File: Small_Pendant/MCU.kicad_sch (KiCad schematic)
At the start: 17 parts, among them U2 SN74LVC1T45DCK

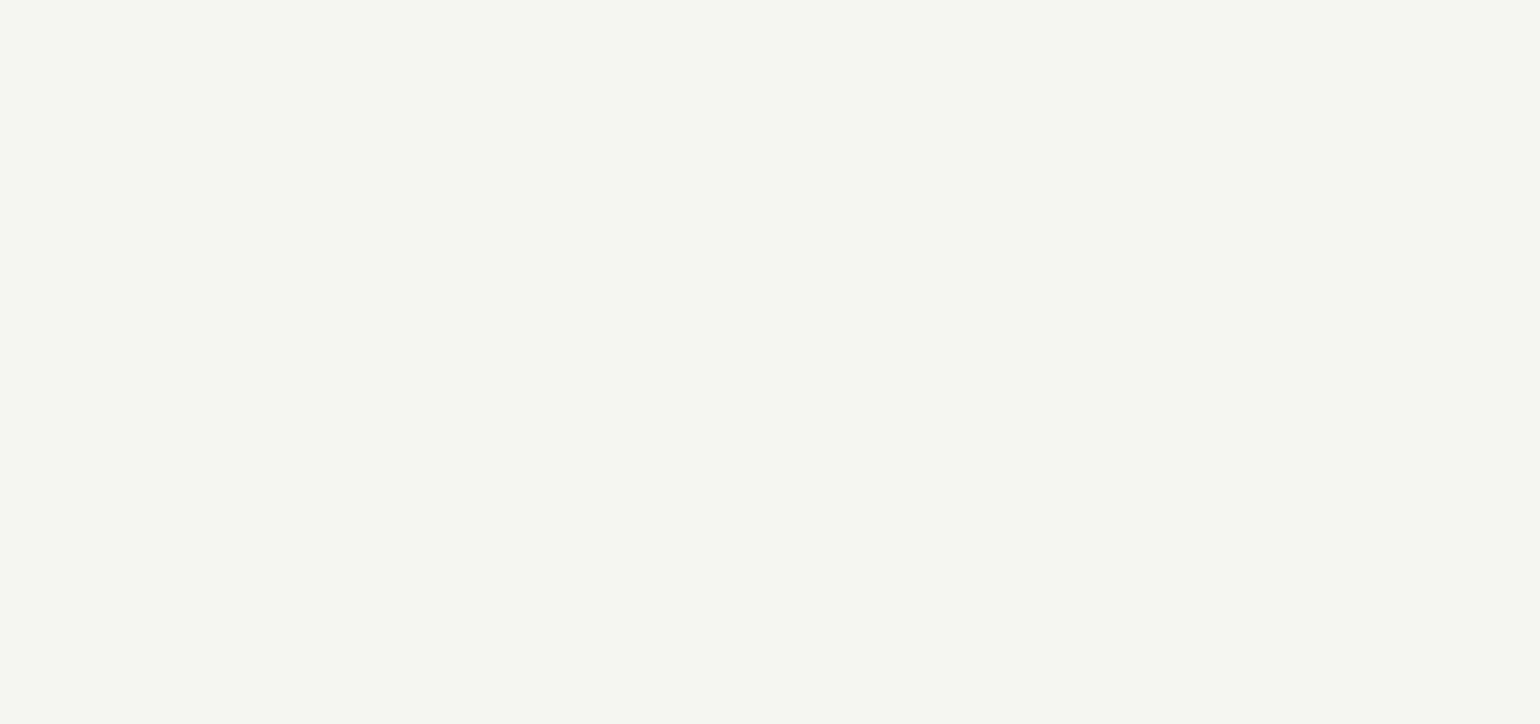
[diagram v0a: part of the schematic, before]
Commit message: [HW] Update TODOs and combine USB Power Rails
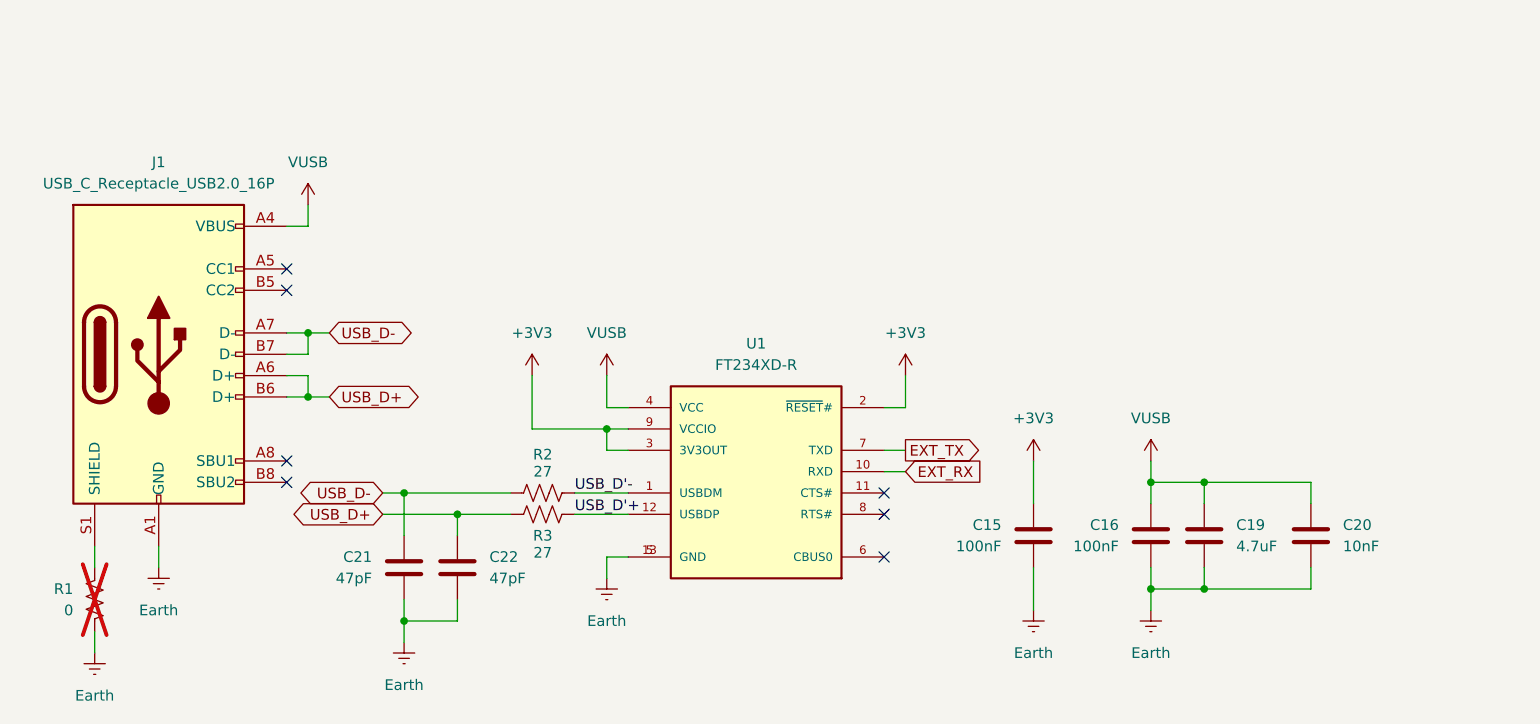
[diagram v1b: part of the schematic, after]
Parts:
- added C15, C16: 100nF, Capacitor_SMD:C_0402_1005Metric, symbol Device:C
- added C19: 4.7uF, Capacitor_SMD:C_0402_1005Metric, symbol Device:C
- added C20: 10nF, Capacitor_SMD:C_0402_1005Metric, symbol Device:C
- added C21, C22: 47pF, Capacitor_SMD:C_0402_1005Metric, symbol Device:C
- added J1: USB_C_Receptacle_USB2.0_16P, Connector_USB:USB_C_Receptacle_GCT_USB4105-xx-A_16P_TopMnt_Horizontal, symbol Connector:USB_C_Receptacle_USB2.0_16P
- added R1: 0, Resistor_SMD:R_0402_1005Metric, symbol Device:R_US
- added R2, R3: 27, Resistor_SMD:R_0402_1005Metric, symbol Device:R_US
- added U1: FT234XD-R, Package_DFN_QFN:DFN-12-1EP_3x3mm_P0.45mm_EP1.65x2.38mm, symbol Interface_USB:FT234XD-R
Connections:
- net +3V3: now also C15.1, U1.2 (~{RESET}#), U1.3 (3V3OUT), U1.9 (VCCIO)
- net Earth: now also C15.2, C16.2, C19.2, C20.2, C21.2, C22.2, J1.A1 (GND), J1.A12 (GND), J1.B1 (GND), J1.B12 (GND), R1.1, U1.13 (GND), U1.5 (GND)
- new net: J1.S1 (SHIELD), R1.2
- new net EXT_RX: U1.10 (RXD)
- new net EXT_TX: U1.7 (TXD)
- new net USB_D'+: R3.2, U1.12 (USBDP)
- new net USB_D'-: R2.2, U1.1 (USBDM)
- new net USB_D+: C22.1, J1.A6 (D+), J1.B6 (D+), R3.1
- new net USB_D-: C21.1, J1.A7 (D-), J1.B7 (D-), R2.1
- new net VUSB: C16.1, C19.1, C20.1, J1.A4 (VBUS), J1.A9 (VBUS), J1.B4 (VBUS), J1.B9 (VBUS), U1.4 (VCC)
- no-connect marks 0 -> 7

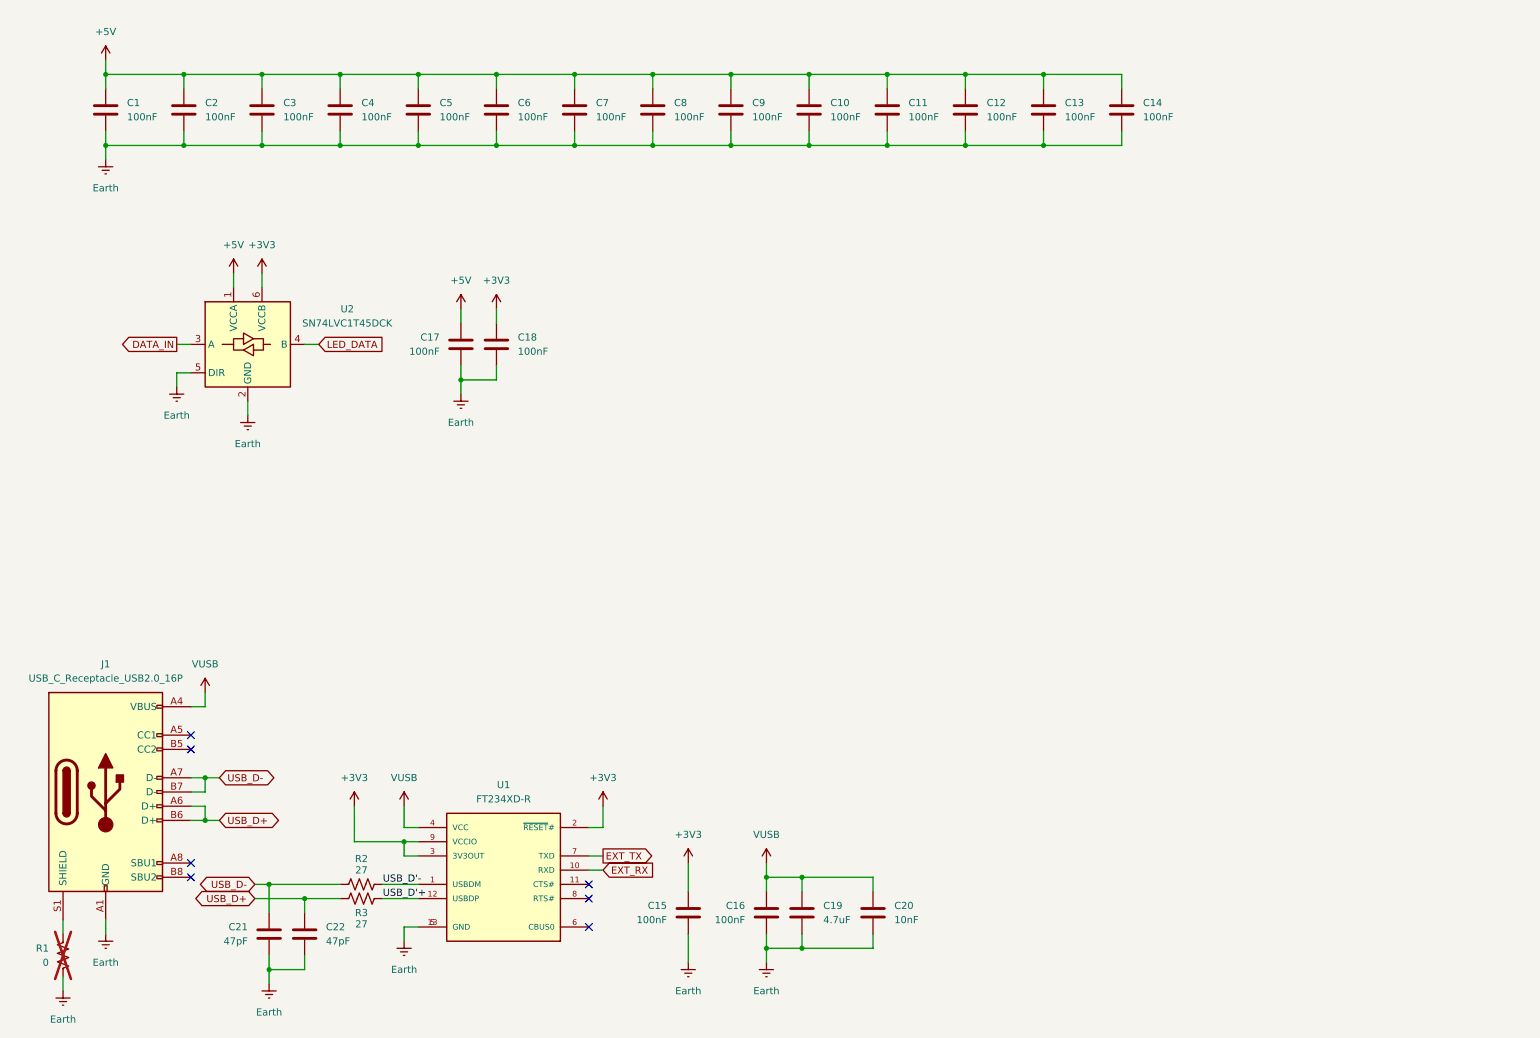
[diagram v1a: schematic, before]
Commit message: [HW] Remove Blind Vias, add 5k1 CC resistors for 5V3A USB-C TODO: 3V3 Regulator (May switch FTDI to that) TODO: MCU (OSC?)
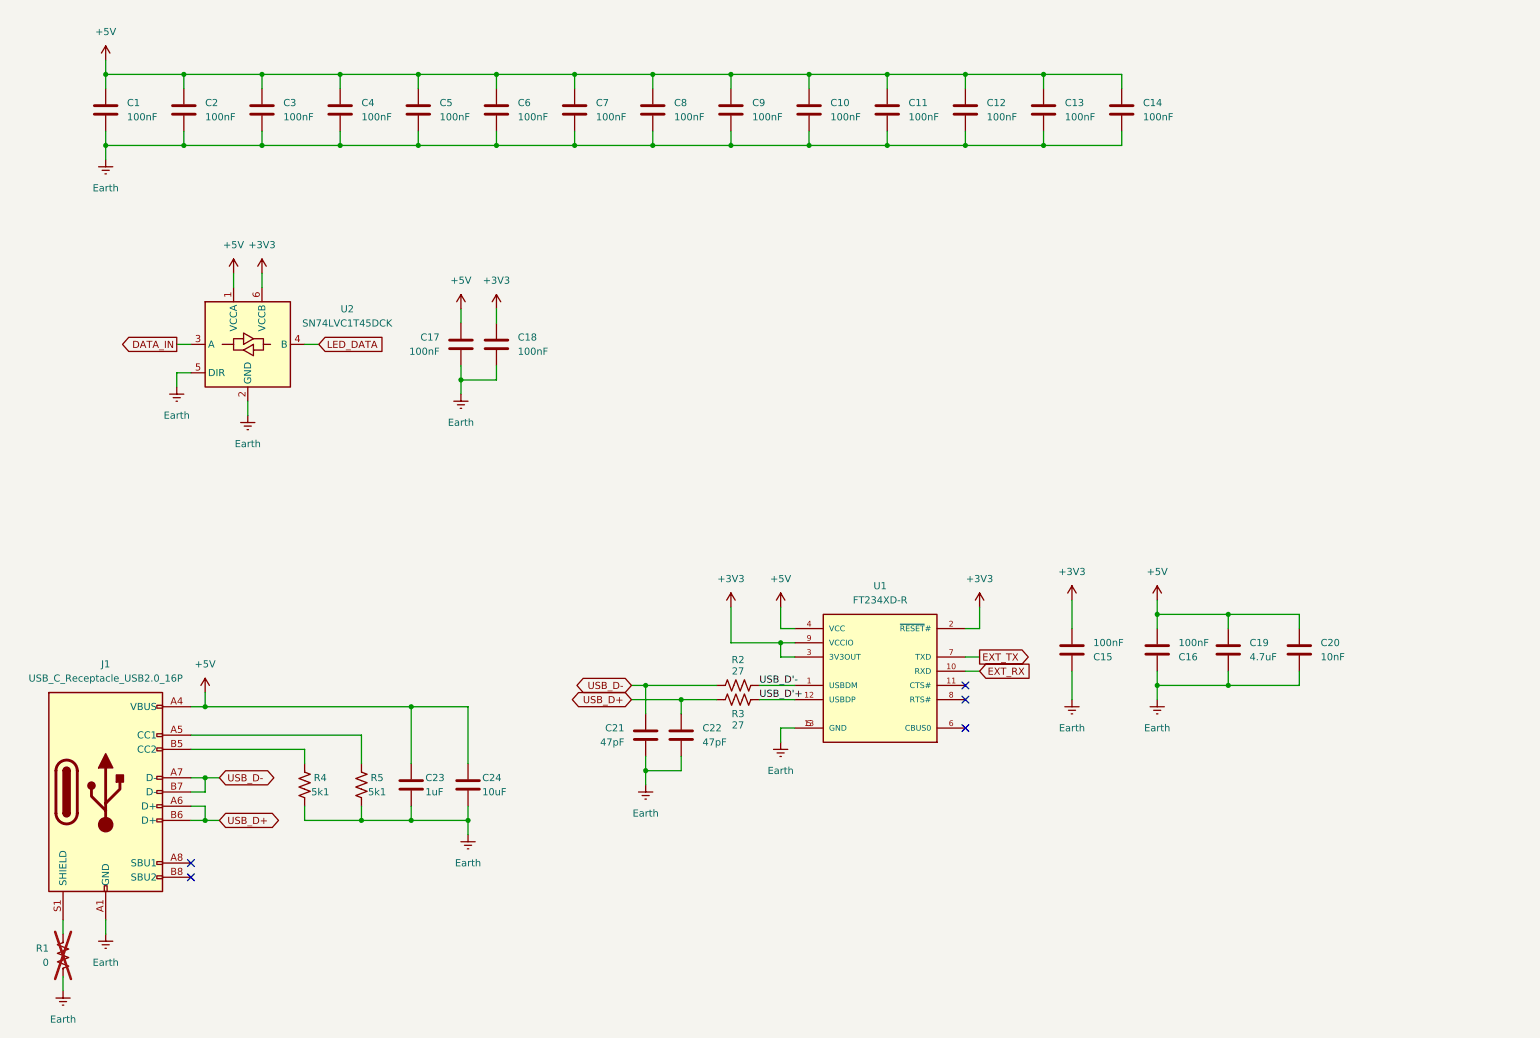
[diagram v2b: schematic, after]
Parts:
- added C23: 1uF, Capacitor_SMD:C_0402_1005Metric, symbol Device:C
- added C24: 10uF, Capacitor_SMD:C_0402_1005Metric, symbol Device:C
- added R4, R5: 5k1, Resistor_SMD:R_0402_1005Metric, symbol Device:R_US
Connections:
- net +3V3: now also C15.2; no longer C15.1
- net +5V: now also C16.2, C19.1, C20.1, J1.A4 (VBUS), J1.A9 (VBUS), J1.B4 (VBUS), J1.B9 (VBUS), U1.4 (VCC), C23.1, C24.1
- net Earth: now also C15.1, C16.1, C23.2, C24.2, R4.2, R5.2; no longer C15.2, C16.2
- net at J1.A5 (CC1): now also R5.1
- net at J1.B5 (CC2): now also R4.1
- removed net VUSB: C16.1, C19.1, C20.1, J1.A4 (VBUS), J1.A9 (VBUS), J1.B4 (VBUS), J1.B9 (VBUS), U1.4 (VCC)
- no-connect marks 7 -> 5
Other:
- moved on the sheet: C15, C16, C19, C20, C21, C22, R2, R3, U1

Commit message: [HW] Split Boards, need to move Caps for LEDs and add all the assorcted stuff for the ESP32
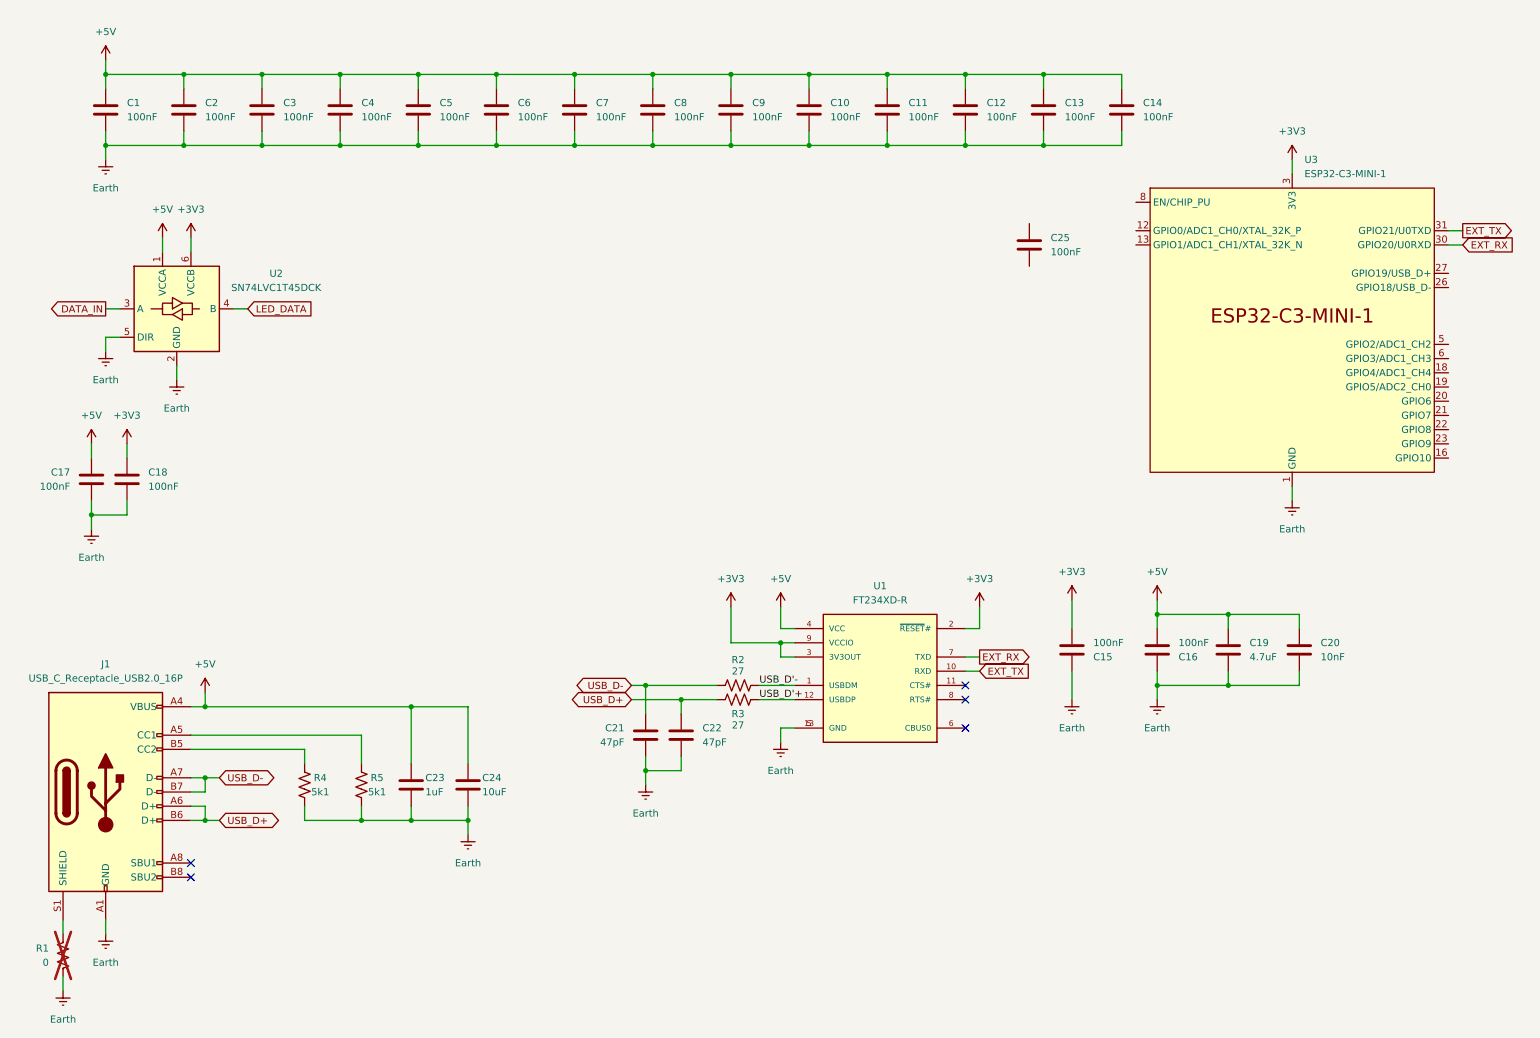
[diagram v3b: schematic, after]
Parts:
- added C25: 100nF, Capacitor_SMD:C_0402_1005Metric, symbol Device:C
- added U3: ESP32-C3-MINI-1, MCU_Espressif_Official:ESP32-C3-MINI-1, symbol MCU_Espressif_Official:ESP32-C3-MINI-1
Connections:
- net +3V3: now also U3.3 (3V3)
- net EXT_RX: now also U1.7 (TXD), U3.30 (GPIO20/U0RXD); no longer U1.10 (RXD)
- net EXT_TX: now also U1.10 (RXD), U3.31 (GPIO21/U0TXD); no longer U1.7 (TXD)
- net Earth: now also U3.1 (GND), U3.11 (GND), U3.14 (GND), U3.2 (GND), U3.36 (GND), U3.37 (GND), U3.38 (GND), U3.39 (GND), U3.40 (GND), U3.41 (GND), U3.42 (GND), U3.43 (GND), U3.44 (GND), U3.45 (GND), U3.46 (GND), U3.47 (GND), U3.48 (GND), U3.49 (GND), U3.50 (GND), U3.51 (GND), U3.52 (GND), U3.53 (GND)
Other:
- moved on the sheet: C17, C18, U2

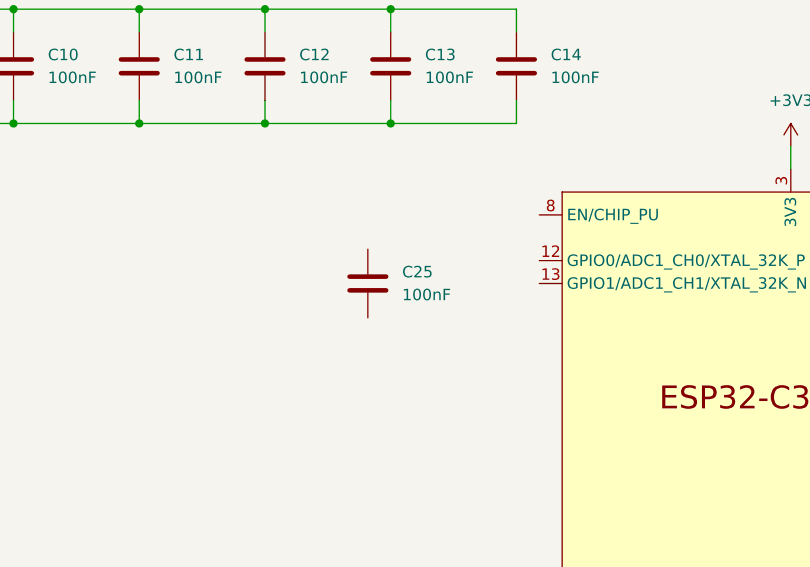
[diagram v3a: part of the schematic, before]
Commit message: [HW] Figure out MCU board shape and add power and ground planes
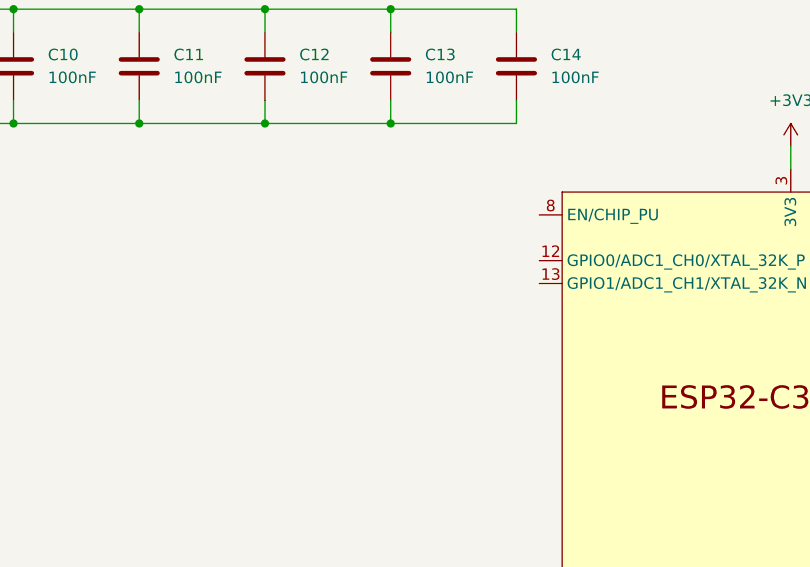
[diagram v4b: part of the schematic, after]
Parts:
- removed C25: 100nF, Capacitor_SMD:C_0402_1005Metric, symbol Device:C
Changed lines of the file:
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@@
-	(symbol
-		(lib_id "Device:C")
-		(at 195.58 55.88 0)
-		(unit 1)
-		(exclude_from_sim no)
-		(in_bom yes)
-		(on_board yes)
-		(dnp no)
-		(fields_autoplaced yes)
-		(property "Reference" "C25"
-			(at 199.39 54.6099 0)
-			(effects
-				(font
-					(size 1.27 1.27)
-				)
-				(justify left)
-			)
-		)
-		(property "Value" "100nF"
-			(at 199.39 57.1499 0)
-			(effects
-				(font
-					(size 1.27 1.27)
-				)
-				(justify left)
-			)
-		)
-		(property "Footprint" "Capacitor_SMD:C_0402_1005Metric"
-			(at 196.5452 59.69 0)
-			(effects
-				(font
-					(size 1.27 1.27)
-				)
-				(hide yes)
-			)
-		)
-		(property "Datasheet" "~"
-			(at 195.58 55.88 0)
-			(effects
-				(font
-					(size 1.27 1.27)
-				)
-				(hide yes)
-			)
-		)
-		(property "Description" "Unpolarized capacitor"
-			(at 195.58 55.88 0)
-			(effects
-				(font
-					(size 1.27 1.27)
-				)
-				(hide yes)
-			)
-		)
-		(pin "1"
-		)
-		(pin "2"
-		)
-		(instances
-			(project "Small_Pendant"
-				(path "/e1f67532-4244-48a0-a633-004c4e91cc2f/14f335fc-598f-404a-bfcd-3d46c6f23e92"
-					(reference "C25")
-					(unit 1)
-				)
-			)
-		)
-	)
 	(symbol
 		(lib_id "Device:C")
